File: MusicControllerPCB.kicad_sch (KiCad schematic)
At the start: 7 parts, among them SW1 SW_Push, SW2 SW_Push, SW3 SW_Push, SW4 SW_Push

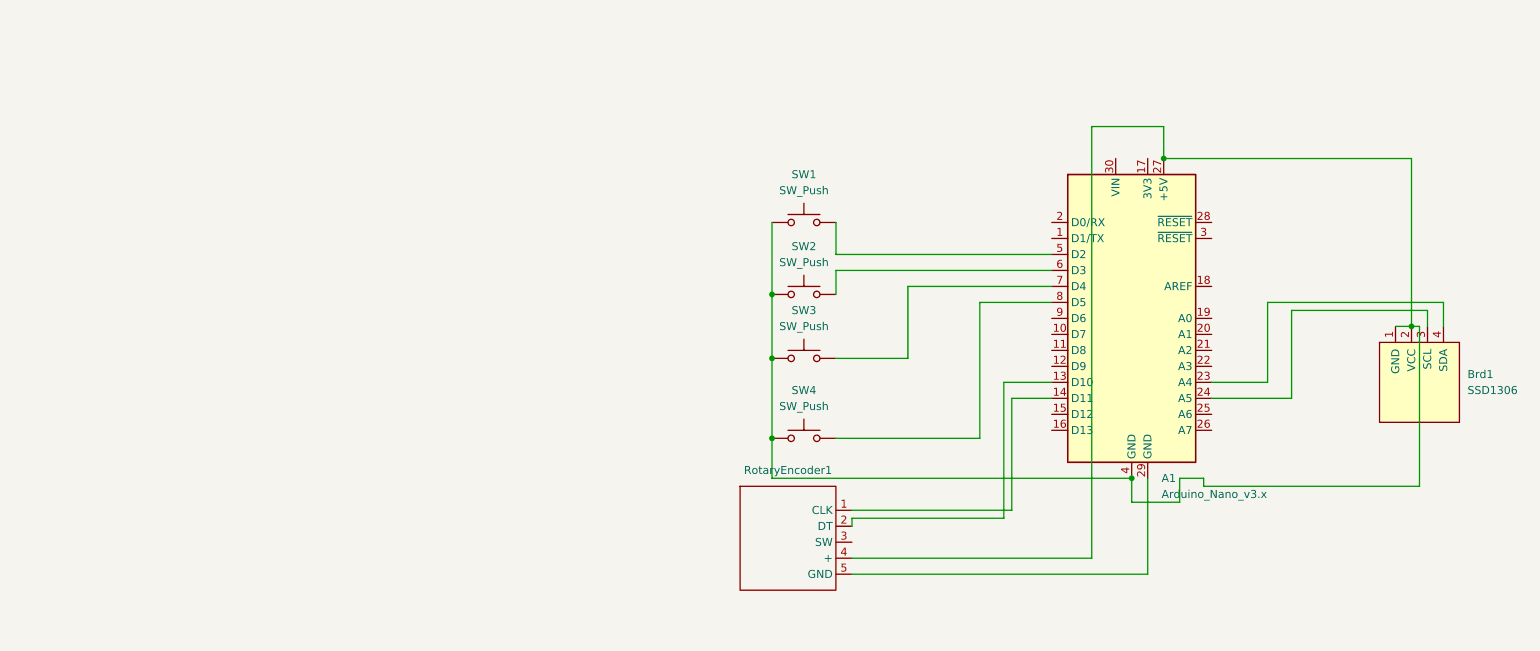
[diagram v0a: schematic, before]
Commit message: Some cleanup
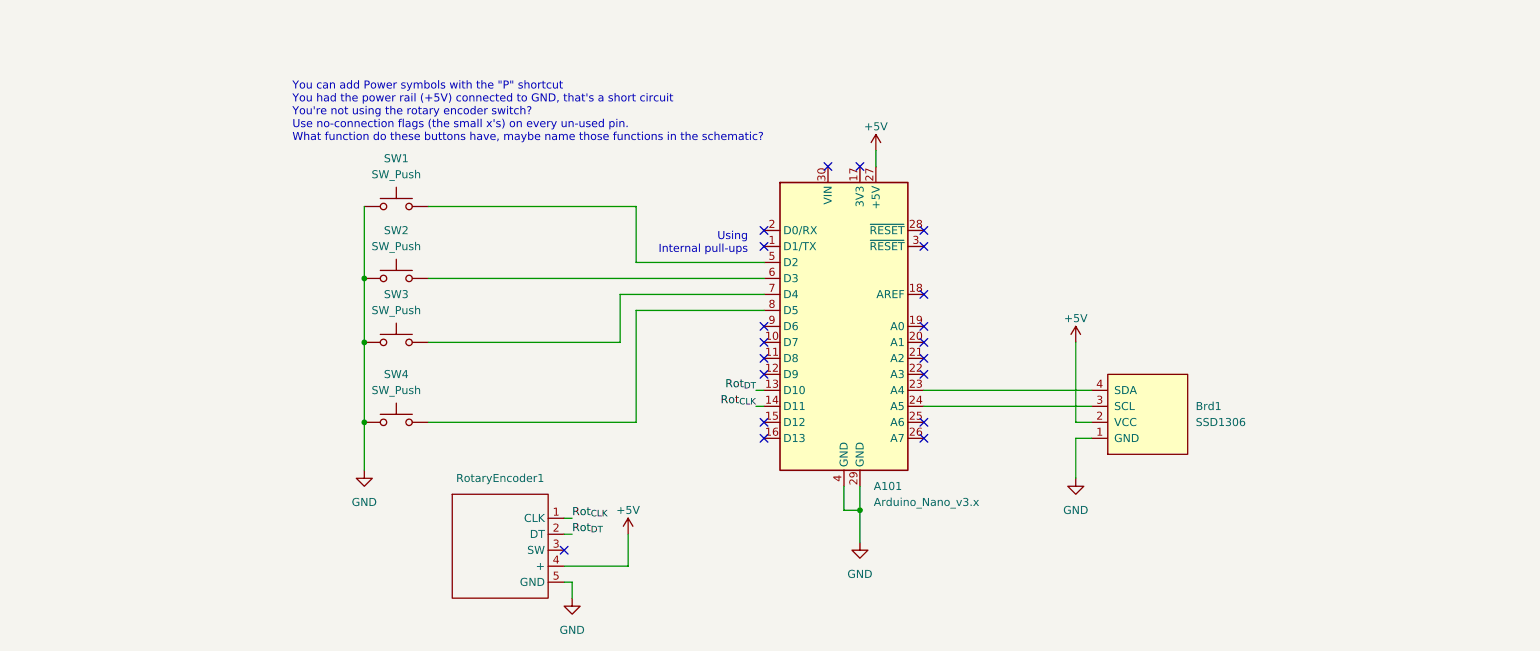
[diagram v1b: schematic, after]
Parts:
- removed A1: Arduino_Nano_v3.x, Module:Arduino_Nano, symbol MCU_Module:Arduino_Nano_v3.x
- added A101: Arduino_Nano_v3.x, Module:Arduino_Nano, symbol _project:Arduino_Nano_v3.x
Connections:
- net Rot_{DT}: now reaches RotaryEncoder1.2 (DT)
- net Rot_{DT}: now also A101.13 (D10)
- net Rot_{CLK}: now reaches RotaryEncoder1.1 (CLK)
- net Rot_{CLK}: now also A101.14 (D11)
- net at Brd1.4 (SDA): now also A101.23 (A4)
- net at Brd1.3 (SCL): now also A101.24 (A5)
- net GND: now reaches Brd1.1 (GND), SW1.1, SW2.1, SW3.1, SW4.1
- net GND: now also RotaryEncoder1.5 (GND), A101.29 (GND), A101.4 (GND); no longer Brd1.2 (VCC), RotaryEncoder1.4 (+)
- net at SW1.2: now also A101.5 (D2)
- net at SW2.2: now also A101.6 (D3)
- net at SW3.2: now also A101.7 (D4)
- net at SW4.2: now also A101.8 (D5)
- new net +5V: A101.27 (+5V), Brd1.2 (VCC), RotaryEncoder1.4 (+)
- no-connect marks 0 -> 20
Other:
- note added: "Using Internal pull-ups"
- note added: "You can add Power symbols with the "P" shortcut You had the power rail (+5V) connected to GND, that's a short circuit You're not using the rotary encoder switch? Use no-connection flags (the small x's) on every un-used pin. What function do these buttons have, maybe name those functions in the schematic?"
- moved on the sheet: Brd1, RotaryEncoder1, SW1, SW2, SW3, SW4

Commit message: Added export
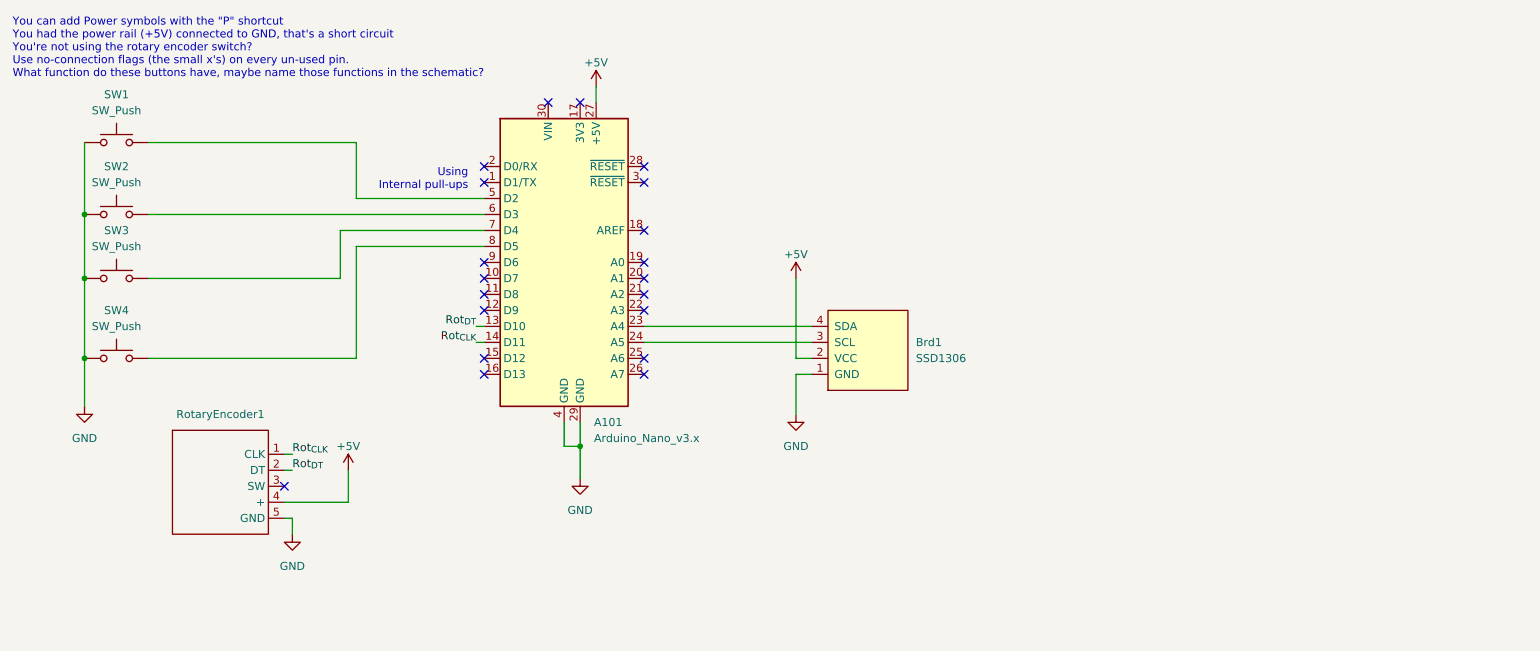
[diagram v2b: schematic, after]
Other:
- title: (none) -> Add some sort of a title?
- moved on the sheet: A101, Brd1, RotaryEncoder1, SW1, SW2, SW3, SW4
